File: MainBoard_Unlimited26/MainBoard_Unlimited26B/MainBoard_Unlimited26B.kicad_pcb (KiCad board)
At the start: 2 copper layers, 95 x 60 mm, 40 parts, among them J1 power, J2 Conn_01x04_Pin, U1 TA6586, U10 TA6586, U2 TA6586, U3 TA6586, U4 TA6586, U5 TA6586, U6 815

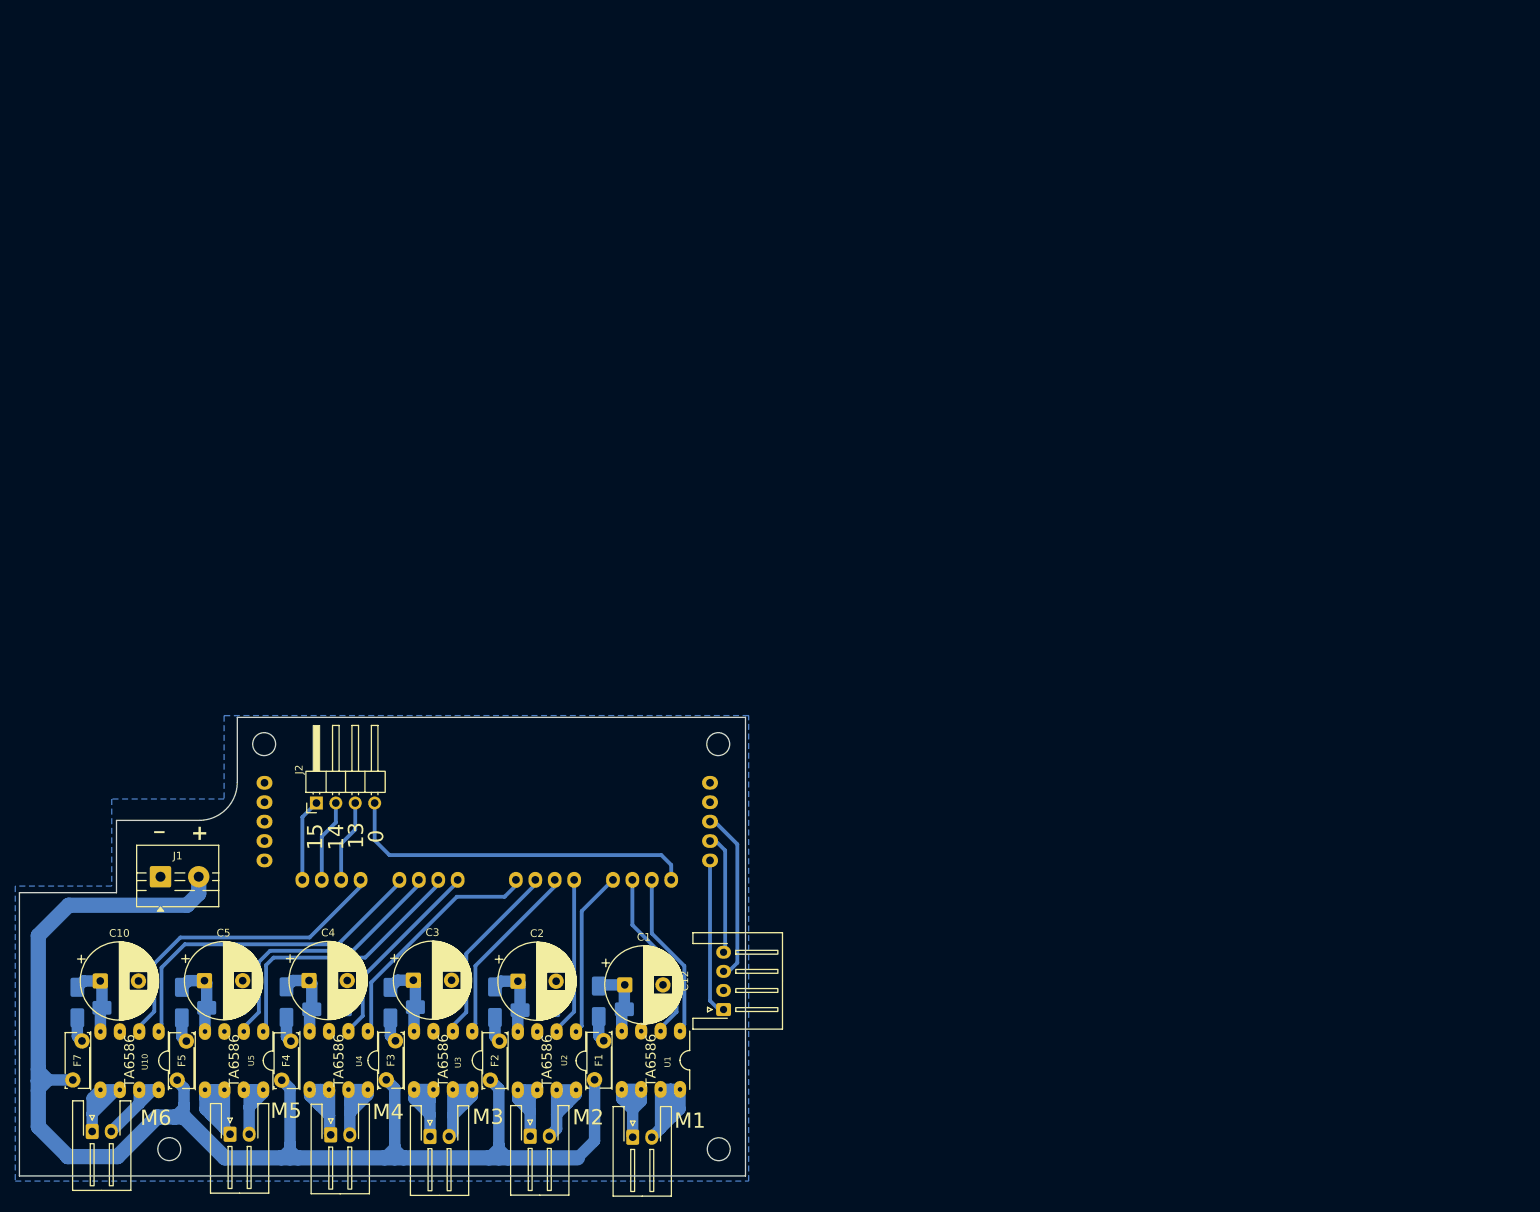
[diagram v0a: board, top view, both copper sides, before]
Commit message: update
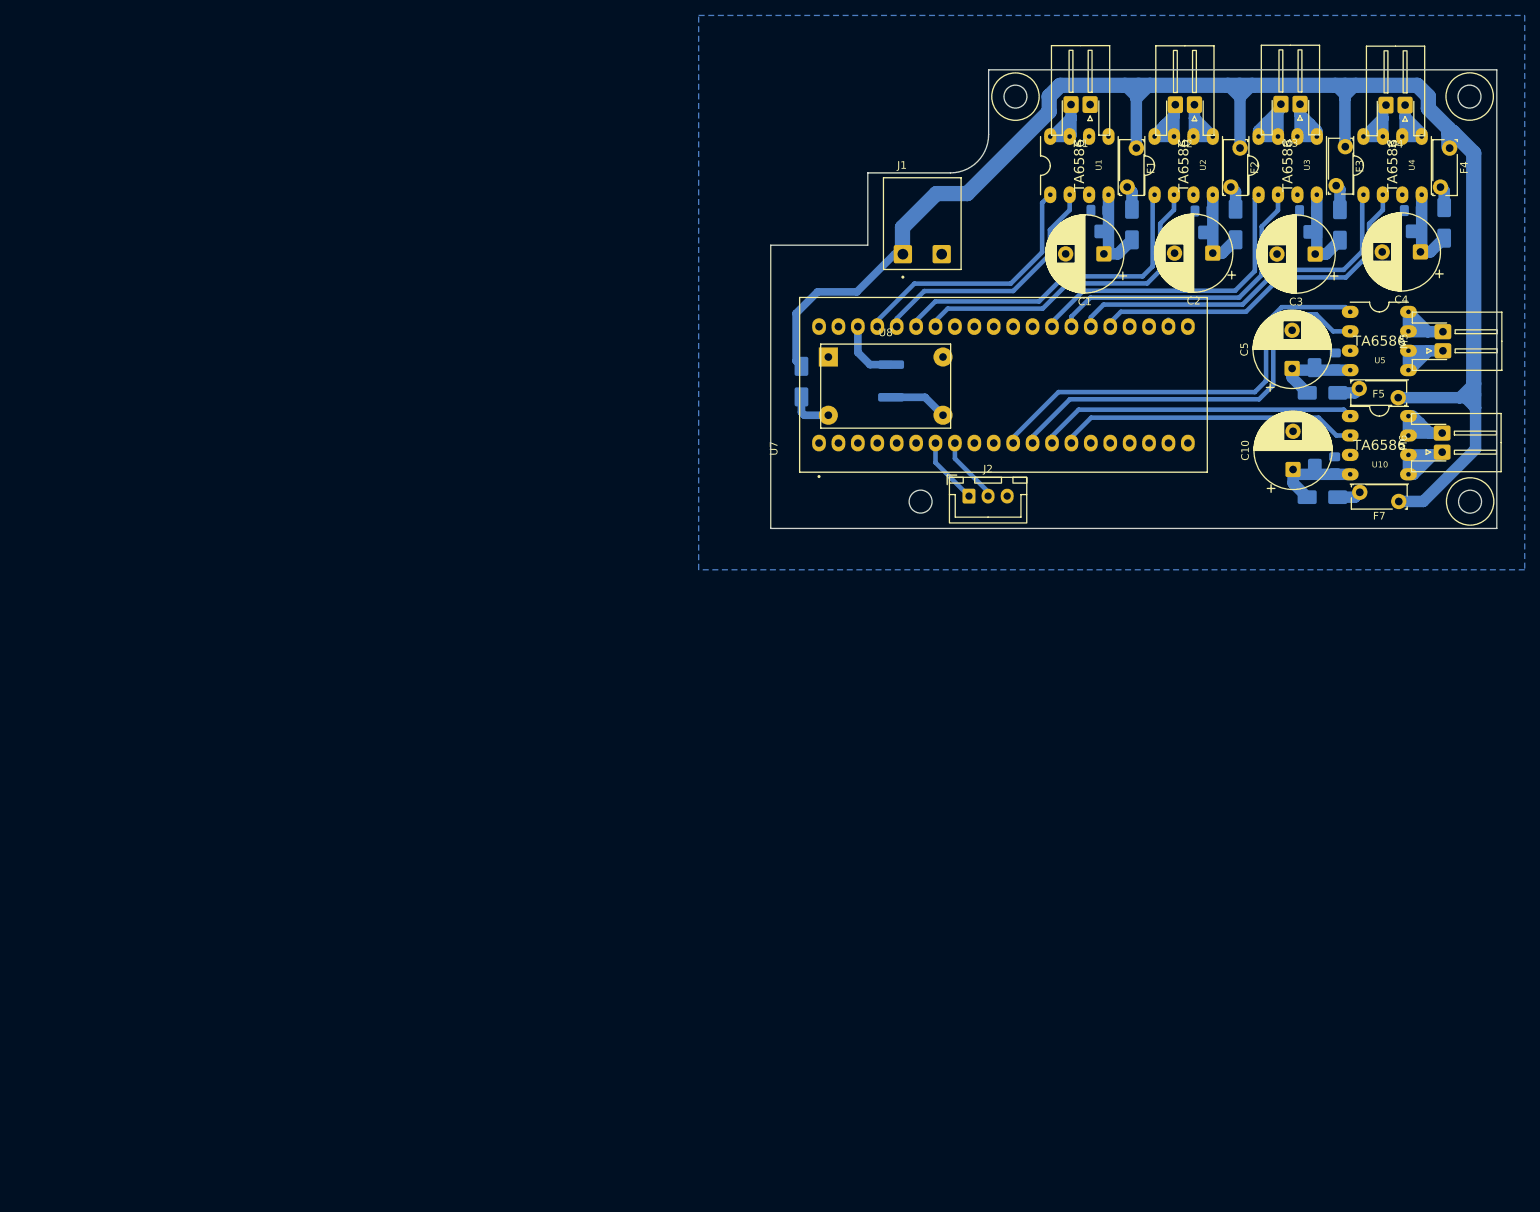
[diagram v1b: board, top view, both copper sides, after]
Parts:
- removed U6: 815, pca:MODULE_815_B
- added C11: 0.1uF, Capacitor_SMD:C_0805_2012Metric_Pad1.18x1.45mm_HandSolder, B.Cu at (236.6, 59.3)
- added C6: 0.1uF, Capacitor_SMD:C_0805_2012Metric_Pad1.18x1.45mm_HandSolder, B.Cu at (205.7, 39.6)
- added C7: 0.1uF, Capacitor_SMD:C_0805_2012Metric_Pad1.18x1.45mm_HandSolder, B.Cu at (219.3, 39.7)
- added C8: 0.1uF, Capacitor_SMD:C_0805_2012Metric_Pad1.18x1.45mm_HandSolder, B.Cu at (233.0, 39.7)
- added C9: 0.1uF, Capacitor_SMD:C_0805_2012Metric_Pad1.18x1.45mm_HandSolder, B.Cu at (246.7, 39.7)
- added D13: D_Schottky, Diode_SMD:D_SMA, B.Cu at (166.8, 62.0)
- added F6: Polyfuse, Fuse:Fuse_1812_4532Metric, B.Cu at (178.5, 62.0)
- added U7: ZC323000, STM blue pill:MODULE_ZC323000, F.Cu at (193.2, 62.5)
- added U8: MP1584_3A_Mini, mp1548:Mini360, F.Cu at (177.8, 62.6)
- C12: value AB conn -> 0.1uF; footprint Connector_JST:JST_XH_S4B-XH-A-1_1x04_P2.50mm_Horizontal -> Capacitor_SMD:C_0805_2012Metric_Pad1.18x1.45mm_HandSolder; moved to B.Cu
- J1: footprint TerminalBlock:TerminalBlock_MaiXu_MX126-5.0-02P_1x02_P5.00mm -> terminal block right angel:TE_282815-2
- J2: value Conn_01x04_Pin -> Conn_01x03_Pin; footprint Connector_PinHeader_2.54mm:PinHeader_1x04_P2.54mm_Horizontal -> Connector_JST:JST_XH_B3B-XH-A_1x03_P2.50mm_Vertical
- moved M6 197.7 mm to (250.6, 71.3), turned to 90 degrees
- moved U4 196.5 mm to (246.6, 24.9), turned to 90 degrees
- moved F4 195.5 mm to (251.6, 31.5), turned to -90 degrees
- moved U10 195.3 mm to (251.3, 72.9), turned to 0 degrees
- moved M4 194.7 mm to (245.7, 25.9), turned to 180 degrees
- moved U5 190.0 mm to (251.3, 59.3), turned to 0 degrees
- moved F7 189.3 mm to (244.9, 77.7), turned to 180 degrees
- moved M5 188.9 mm to (250.7, 58.0), turned to 90 degrees
- moved F5 183.0 mm to (244.8, 64.2), turned to 180 degrees
- moved D4 178.7 mm to (250.8, 41.3), turned to 90 degrees
- moved U3 177.6 mm to (232.9, 24.9), turned to 90 degrees
- moved D9 177.2 mm to (245.1, 42.4), turned to 180 degrees
- moved M3 176.6 mm to (232.0, 25.8), turned to 180 degrees
- moved D11 175.8 mm to (234.9, 77.2), turned to 0 degrees
- moved F3 175.1 mm to (237.9, 31.3), turned to -90 degrees
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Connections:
- C12 pad 1: +3.3V -> Net-(D11-K)
- D10 pad 2: Net-(D10-A) -> GND
- D2 pad 2: GND -> Net-(D2-A)
- D3 pad 2: GND -> Net-(D3-A)
- D4 pad 2: GND -> Net-(D4-A)
- D5 pad 2: GND -> Net-(D5-A)
- D7 pad 2: Net-(D7-A) -> GND
- D8 pad 2: Net-(D8-A) -> GND
- D9 pad 2: Net-(D9-A) -> GND
- F2 pad 2: Net-(D7-A) -> Net-(D2-A)
- F3 pad 2: Net-(D8-A) -> Net-(D3-A)
- F4 pad 2: Net-(D9-A) -> Net-(D4-A)
- F5 pad 2: Net-(D10-A) -> Net-(D5-A)
- J1 pad 1: GND -> +12V
- J1 pad 2: +12V -> GND
- J2 pad 1: PCA15 -> TX
- J2 pad 2: PCA14 -> RX
- J2 pad 3: PCA13 -> GND
- U1 pad BI: PCA1 -> PB9
- U1 pad FI: PCA2 -> PB8
- U10 pad BI: PCA11 -> PB0
- U10 pad FI: PCA12 -> PB1
- U2 pad BI: PCA3 -> PB7
- U2 pad FI: PCA4 -> PB6
- U3 pad BI: PCA5 -> PA11
- U3 pad FI: PCA6 -> PA10
- U4 pad BI: PCA7 -> PA9
- U4 pad FI: PCA8 -> PA8
- U5 pad BI: PCA9 -> PA6
- U5 pad FI: PCA10 -> PA7
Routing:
- net PA6: track 0.00 -> 56.6 mm
- net PA7: track 0.00 -> 54.5 mm
- net PA9: track 0.00 -> 47.8 mm
- net PCA0: track 47.0 -> 0.00 mm
- net PA8: track 0.00 -> 46.6 mm
- net PCA11: track 44.6 -> 0.00 mm
- net PB7: track 0.00 -> 44.1 mm
- net PB6: track 0.00 -> 43.5 mm
- net PCA12: track 41.8 -> 0.00 mm
- net PB0: track 0.00 -> 41.7 mm
- net PA11: track 0.00 -> 40.1 mm
- net PA10: track 0.00 -> 39.8 mm
- net PB1: track 0.00 -> 39.3 mm
- net PCA9: track 36.3 -> 0.00 mm
- net PCA10: track 35.7 -> 0.00 mm
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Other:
- board text removed: "+"
- board text removed: "0"
- board text removed: "13"
- board text removed: "14"
- board text removed: "15"
- board text removed: "_"
